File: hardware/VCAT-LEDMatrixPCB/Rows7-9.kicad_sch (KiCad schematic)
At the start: 54 parts

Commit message: Layout 50% done
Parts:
- C55, C56, C57, C58, C59, C60, C61, C62, C63, C64, C65, C66, C67, C68, C69, C70, C71, C72, C73, C74, C75, C76, C77, C78, C79, C80, C81: footprint Capacitor_SMD:C_0603_1608Metric_Pad1.08x0.95mm_HandSolder -> Capacitor_SMD:C_0603_1608Metric
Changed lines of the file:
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@@
 			)
 		)
-		(property "Footprint" "Capacitor_SMD:C_0603_1608Metric_Pad1.08x0.95mm_HandSolder"
+		(property "Footprint" "Capacitor_SMD:C_0603_1608Metric"
 			(at 119.0752 115.57 0)
 			(effects
@@
 			)
 		)
-		(property "Footprint" "Capacitor_SMD:C_0603_1608Metric_Pad1.08x0.95mm_HandSolder"
+		(property "Footprint" "Capacitor_SMD:C_0603_1608Metric"
 			(at 72.7202 80.01 0)
 			(effects
@@
 			)
 		)
-		(property "Footprint" "Capacitor_SMD:C_0603_1608Metric_Pad1.08x0.95mm_HandSolder"
+		(property "Footprint" "Capacitor_SMD:C_0603_1608Metric"
 			(at 187.6552 116.205 0)
 			(effects
@@
 			)
 		)
-		(property "Footprint" "Capacitor_SMD:C_0603_1608Metric_Pad1.08x0.95mm_HandSolder"
+		(property "Footprint" "Capacitor_SMD:C_0603_1608Metric"
 			(at 233.3752 116.205 0)
 			(effects
@@
 			)
 		)
-		(property "Footprint" "Capacitor_SMD:C_0603_1608Metric_Pad1.08x0.95mm_HandSolder"
+		(property "Footprint" "Capacitor_SMD:C_0603_1608Metric"
 			(at 122.2502 44.45 0)
 			(effects
@@
 			)
 		)
-		(property "Footprint" "Capacitor_SMD:C_0603_1608Metric_Pad1.08x0.95mm_HandSolder"
+		(property "Footprint" "Capacitor_SMD:C_0603_1608Metric"
 			(at 164.1602 80.645 0)
 			(effects
@@
 			)
 		)
-		(property "Footprint" "Capacitor_SMD:C_0603_1608Metric_Pad1.08x0.95mm_HandSolder"
+		(property "Footprint" "Capacitor_SMD:C_0603_1608Metric"
 			(at 73.3552 115.57 0)
 			(effects
@@
 			)
 		)
-		(property "Footprint" "Capacitor_SMD:C_0603_1608Metric_Pad1.08x0.95mm_HandSolder"
+		(property "Footprint" "Capacitor_SMD:C_0603_1608Metric"
 			(at 145.1102 45.085 0)
 			(effects
@@
 			)
 		)
-		(property "Footprint" "Capacitor_SMD:C_0603_1608Metric_Pad1.08x0.95mm_HandSolder"
+		(property "Footprint" "Capacitor_SMD:C_0603_1608Metric"
 			(at 76.5302 44.45 0)
 			(effects
@@
 			)
 		)
-		(property "Footprint" "Capacitor_SMD:C_0603_1608Metric_Pad1.08x0.95mm_HandSolder"
+		(property "Footprint" "Capacitor_SMD:C_0603_1608Metric"
 			(at 213.6902 45.085 0)
 			(effects
@@
 			)
 		)
-		(property "Footprint" "Capacitor_SMD:C_0603_1608Metric_Pad1.08x0.95mm_HandSolder"
+		(property "Footprint" "Capacitor_SMD:C_0603_1608Metric"
 			(at 190.8302 45.085 0)
 			(effects
@@
 			)
 		)
-		(property "Footprint" "Capacitor_SMD:C_0603_1608Metric_Pad1.08x0.95mm_HandSolder"
+		(property "Footprint" "Capacitor_SMD:C_0603_1608Metric"
 			(at 236.5502 45.085 0)
 			(effects
@@
 			)
 		)
-		(property "Footprint" "Capacitor_SMD:C_0603_1608Metric_Pad1.08x0.95mm_HandSolder"
+		(property "Footprint" "Capacitor_SMD:C_0603_1608Metric"
 			(at 53.6702 44.45 0)
 			(effects
@@
 			)
 		)
-		(property "Footprint" "Capacitor_SMD:C_0603_1608Metric_Pad1.08x0.95mm_HandSolder"
+		(property "Footprint" "Capacitor_SMD:C_0603_1608Metric"
 			(at 49.8602 80.01 0)
 			(effects
@@
 			)
 		)
-		(property "Footprint" "Capacitor_SMD:C_0603_1608Metric_Pad1.08x0.95mm_HandSolder"
+		(property "Footprint" "Capacitor_SMD:C_0603_1608Metric"
 			(at 141.3002 80.645 0)
 			(effects
@@
 			)
 		)
-		(property "Footprint" "Capacitor_SMD:C_0603_1608Metric_Pad1.08x0.95mm_HandSolder"
+		(property "Footprint" "Capacitor_SMD:C_0603_1608Metric"
 			(at 209.8802 80.645 0)
 			(effects
@@
 			)
 		)
-		(property "Footprint" "Capacitor_SMD:C_0603_1608Metric_Pad1.08x0.95mm_HandSolder"
+		(property "Footprint" "Capacitor_SMD:C_0603_1608Metric"
 			(at 99.3902 44.45 0)
 			(effects
@@
 			)
 		)
-		(property "Footprint" "Capacitor_SMD:C_0603_1608Metric_Pad1.08x0.95mm_HandSolder"
+		(property "Footprint" "Capacitor_SMD:C_0603_1608Metric"
 			(at 210.5152 116.205 0)
 			(effects
@@
 			)
 		)
-		(property "Footprint" "Capacitor_SMD:C_0603_1608Metric_Pad1.08x0.95mm_HandSolder"
+		(property "Footprint" "Capacitor_SMD:C_0603_1608Metric"
 			(at 50.4952 115.57 0)
 			(effects
@@
 			)
 		)
-		(property "Footprint" "Capacitor_SMD:C_0603_1608Metric_Pad1.08x0.95mm_HandSolder"
+		(property "Footprint" "Capacitor_SMD:C_0603_1608Metric"
 			(at 118.4402 80.01 0)
 			(effects
@@
 			)
 		)
-		(property "Footprint" "Capacitor_SMD:C_0603_1608Metric_Pad1.08x0.95mm_HandSolder"
+		(property "Footprint" "Capacitor_SMD:C_0603_1608Metric"
 			(at 232.7402 80.645 0)
 			(effects
@@
 			)
 		)
-		(property "Footprint" "Capacitor_SMD:C_0603_1608Metric_Pad1.08x0.95mm_HandSolder"
+		(property "Footprint" "Capacitor_SMD:C_0603_1608Metric"
 			(at 167.9702 45.085 0)
 			(effects
@@
 			)
 		)
-		(property "Footprint" "Capacitor_SMD:C_0603_1608Metric_Pad1.08x0.95mm_HandSolder"
+		(property "Footprint" "Capacitor_SMD:C_0603_1608Metric"
 			(at 95.5802 80.01 0)
 			(effects
@@
 			)
 		)
-		(property "Footprint" "Capacitor_SMD:C_0603_1608Metric_Pad1.08x0.95mm_HandSolder"
+		(property "Footprint" "Capacitor_SMD:C_0603_1608Metric"
 			(at 96.2152 115.57 0)
 			(effects
@@
 			)
 		)
-		(property "Footprint" "Capacitor_SMD:C_0603_1608Metric_Pad1.08x0.95mm_HandSolder"
+		(property "Footprint" "Capacitor_SMD:C_0603_1608Metric"
 			(at 187.0202 80.645 0)
 			(effects
@@
 			)
 		)
-		(property "Footprint" "Capacitor_SMD:C_0603_1608Metric_Pad1.08x0.95mm_HandSolder"
+		(property "Footprint" "Capacitor_SMD:C_0603_1608Metric"
 			(at 141.9352 116.205 0)
 			(effects
@@
 			)
 		)
-		(property "Footprint" "Capacitor_SMD:C_0603_1608Metric_Pad1.08x0.95mm_HandSolder"
+		(property "Footprint" "Capacitor_SMD:C_0603_1608Metric"
 			(at 164.7952 116.205 0)
 			(effects

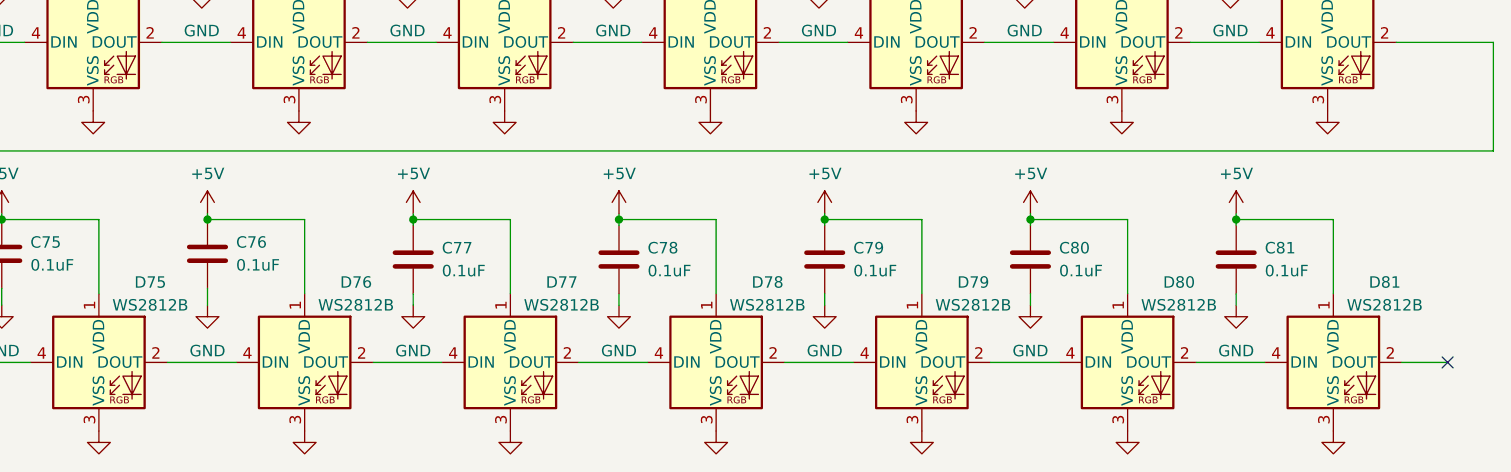
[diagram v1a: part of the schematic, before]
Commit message: Layout Review
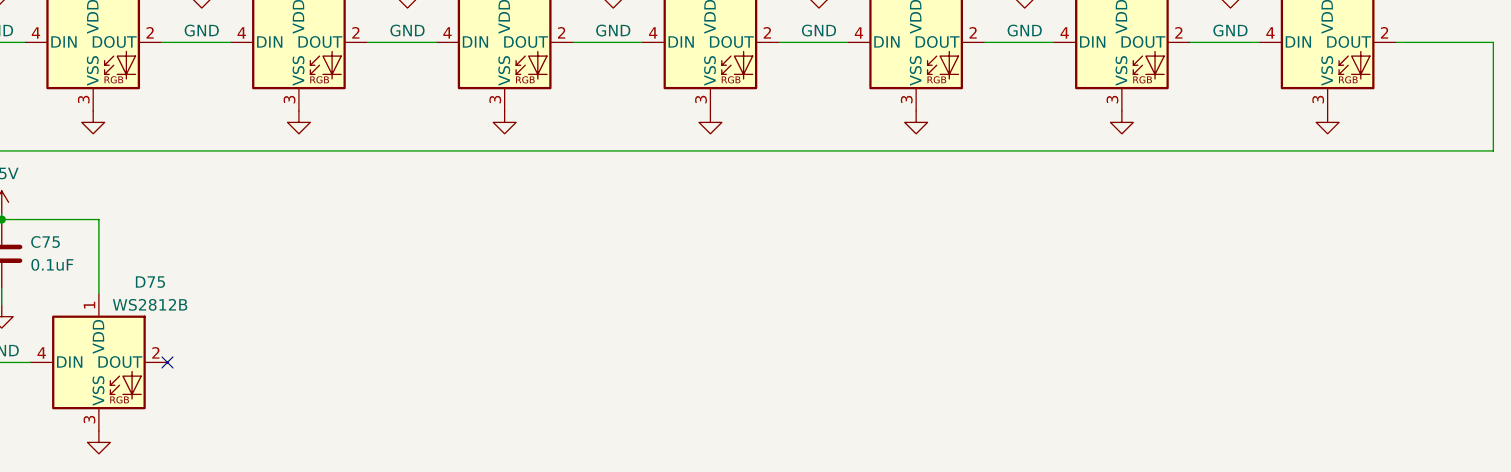
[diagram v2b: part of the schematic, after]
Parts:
- removed C76, C77, C78, C79, C80, C81: 0.1uF, Capacitor_SMD:C_0603_1608Metric, symbol Device:C
- removed D76, D77, D78, D79, D80, D81: WS2812B, LED_SMD:LED_WS2812B_PLCC4_5.0x5.0mm_P3.2mm, symbol LED:WS2812B
